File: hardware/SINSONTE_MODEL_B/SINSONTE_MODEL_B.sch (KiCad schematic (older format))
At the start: 35 parts, among them J1 BAT, J10 Conn_01x02_Male, J11 Conn_01x02_Male, J12 Conn_01x02_Male, J13 Conn_01x02_Male, J14 Conn_01x02_Male, J15 Conn_01x02_Male, J16 Conn_01x02_Male, J17 Conn_01x02_Male, J18 Conn_01x02_Male, J2 CLOCK, J3 PROG, J4 LIGHT_SENSOR, J5 Conn_01x20_Male, J6 Conn_01x20_Male, J7 Conn_01x05_Male, J8 Conn_01x05_Male, J9 Conn_01x02_Male, Q1 2N7000, Q2 PN2222A, SW1 SW_Push, U1 Pico

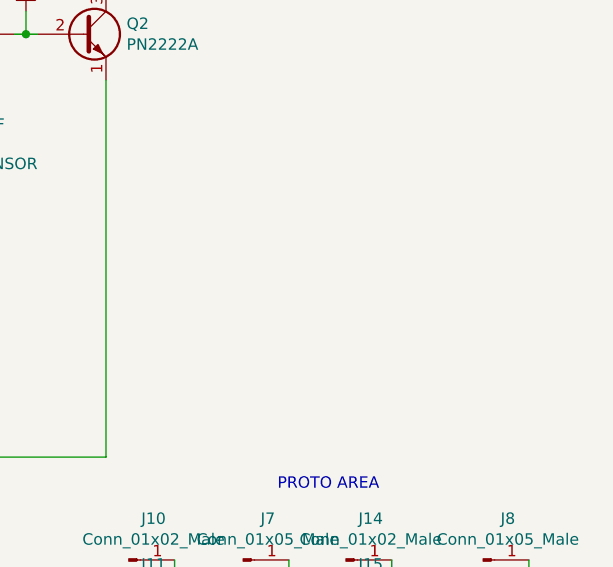
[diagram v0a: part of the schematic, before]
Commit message: shrinkikng in process
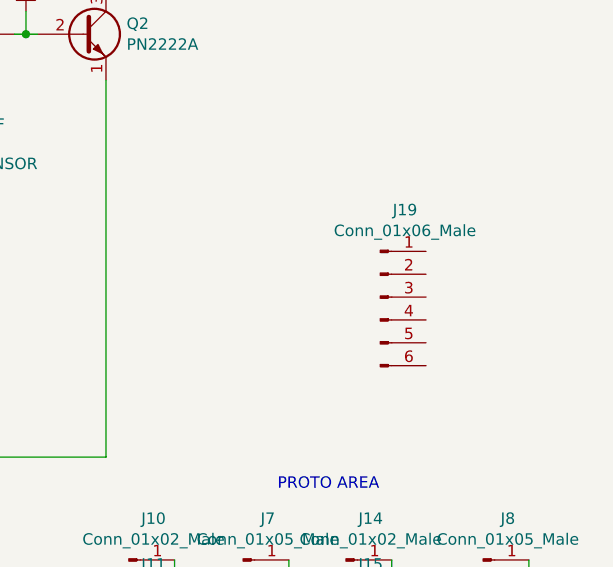
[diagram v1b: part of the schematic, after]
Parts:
- added J19: Conn_01x06_Male, Connector_PinHeader_2.54mm:PinHeader_1x06_P2.54mm_Vertical, symbol Connector:Conn_01x06_Male
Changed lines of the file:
@@
 Text Notes 9750 5150 0    50   ~ 0
 PROTO AREA
+$Comp
+L Connector:Conn_01x06_Male J19
+U 1 1 618C77ED
+P 10200 4300
+F 0 "J19" H 10308 4681 50  0000 C CNN
+F 1 "Conn_01x06_Male" H 10308 4590 50  0000 C CNN
+F 2 "Connector_PinHeader_2.54mm:PinHeader_1x06_P2.54mm_Vertical" H 10200 4300 50  0001 C CNN
+F 3 "~" H 10200 4300 50  0001 C CNN
+	1    10200 4300
+	1    0    0    -1
+$EndComp
 $EndSCHEMATC
